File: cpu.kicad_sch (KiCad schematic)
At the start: 28 parts, among them J81 Conn_01x03_Pin, J82 Conn_Coaxial, J83 Conn_Coaxial, J84 Conn_01x02_Pin, SW81 SW_Push, SW82 SW_Push, U8 ESP32-C6-MINI-1U, U81 74HC595, U82 74HC595, U84 ISOW7842

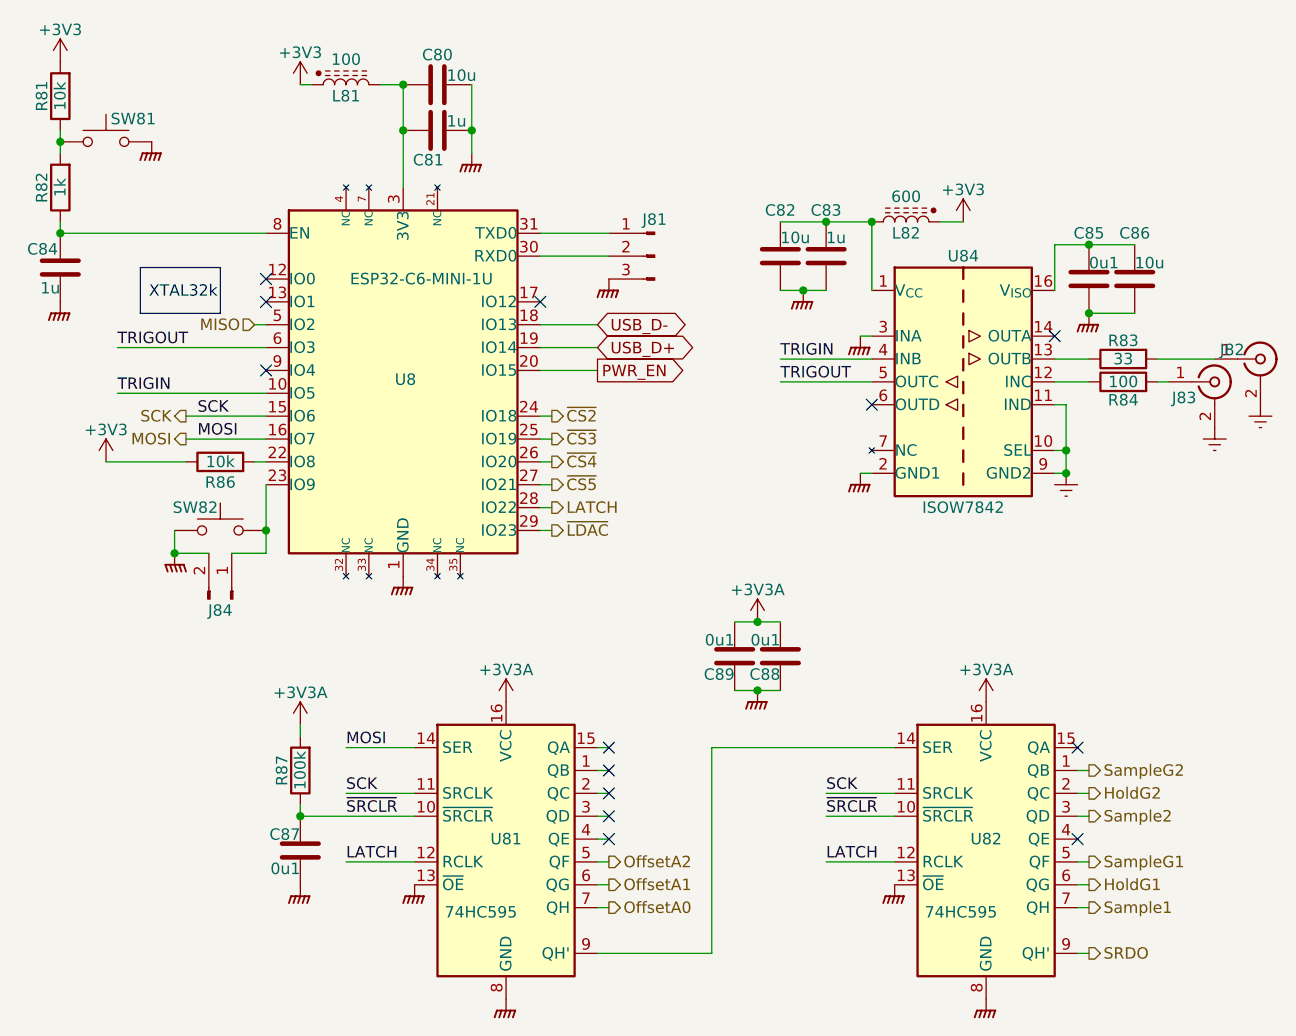
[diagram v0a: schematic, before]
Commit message: Progress checkin.  About to redo FDA feedback again.
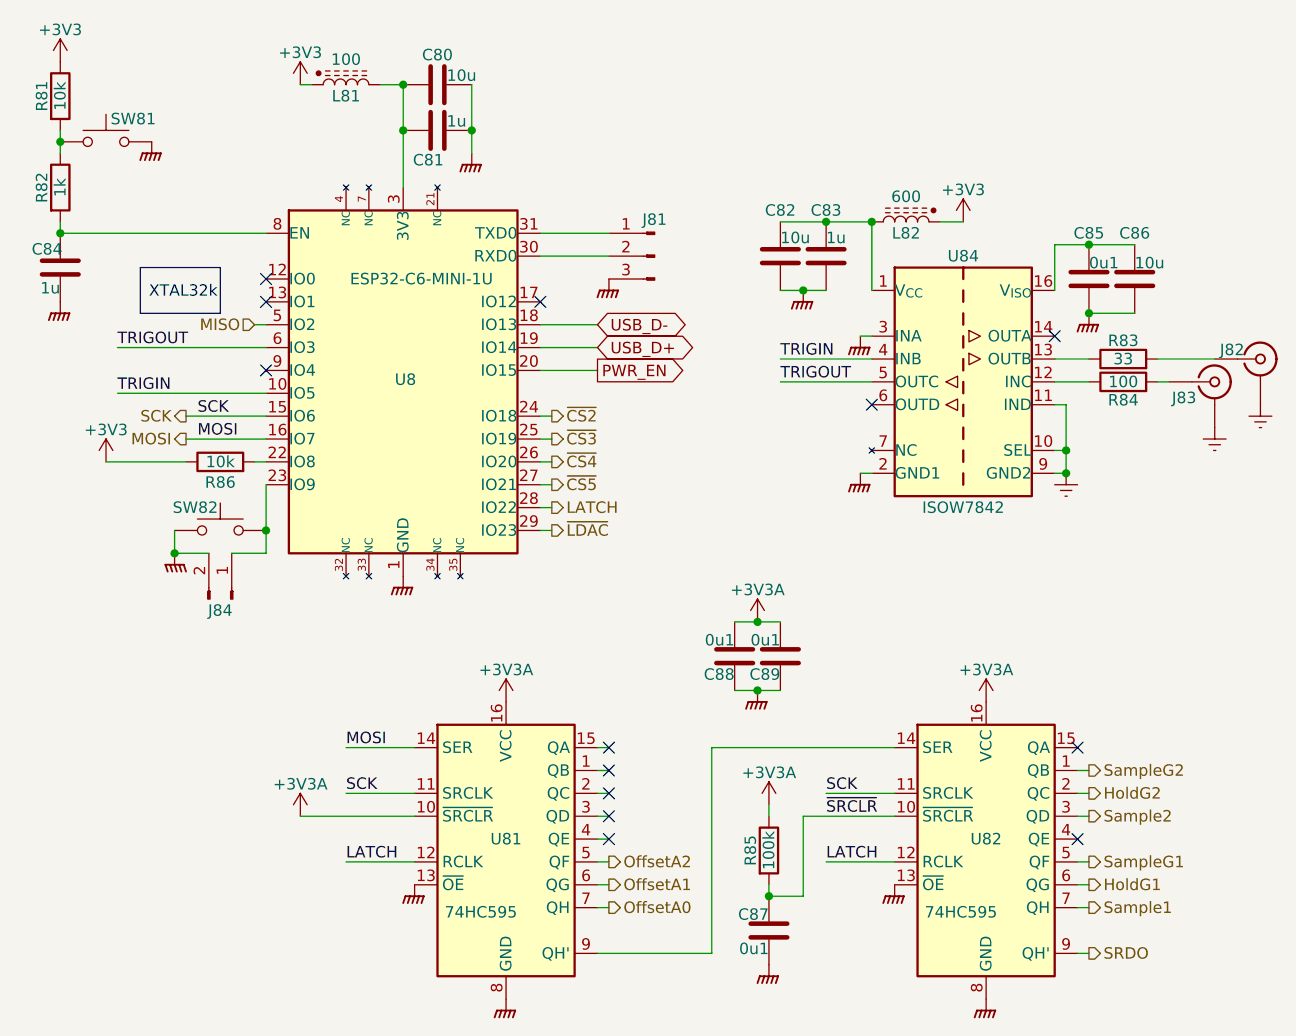
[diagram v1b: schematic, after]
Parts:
- renumbered R87 to R85
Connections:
- net +3V3: now also R81.1; no longer R81.2
- net +3V3A: now also R85.1, U81.10 (~{SRCLR}); no longer R85.2
- net ~{SRCLR}: now also R85.2; no longer R85.1, U81.10 (~{SRCLR})
- net at C84.1, U8.8 (EN): now also R82.2; no longer R82.1
- new net: R81.2, R82.1, SW81.1
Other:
- moved on the sheet: C87, C88, C89, R81, R82, R85
